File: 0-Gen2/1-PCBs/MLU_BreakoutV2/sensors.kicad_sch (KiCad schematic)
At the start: 6 parts, among them U2 MCP9808_MSOP, U3 MCP9808_MSOP, U4 BME280

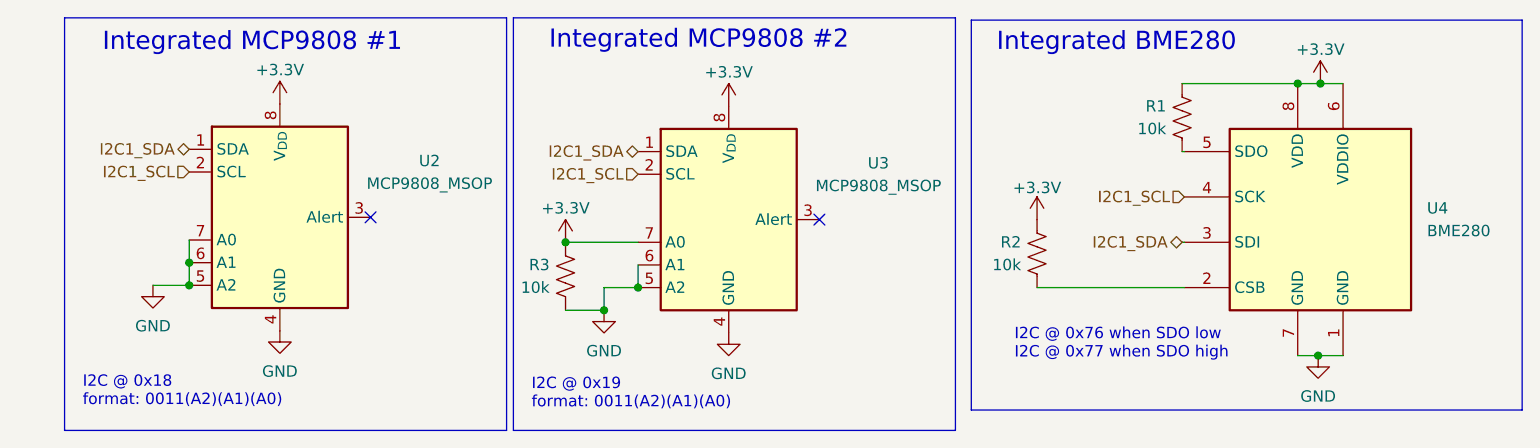
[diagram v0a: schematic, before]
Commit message: before restructure
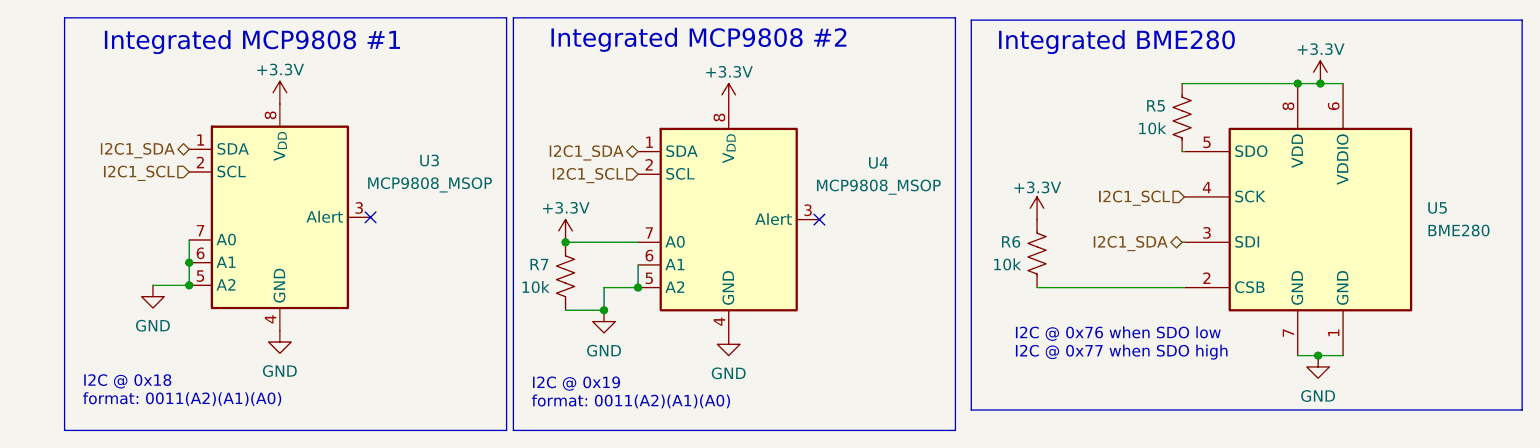
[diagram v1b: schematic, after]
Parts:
- renumbered R1 to R5, R2 to R6, R3 to R7, U2 to U3, U3 to U4, U4 to U5
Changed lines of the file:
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@@
 		(dnp no)
 		(fields_autoplaced yes)
-		(property "Reference" "#PWR021"
+		(property "Reference" "#PWR0145"
 			(at 93.472 59.182 0)
 			(effects
@@
 			(project "MLU_BreakoutV2"
 				(path "/55121ba7-5d22-4fe3-93aa-7f76d75b410c/9dab6a9b-c343-4374-86a4-2dd37d3a47bf"
-					(reference "#PWR021")
+					(reference "#PWR0145")
 					(unit 1)
 				)
@@
 		(dnp no)
 		(fields_autoplaced yes)
-		(property "Reference" "#PWR019"
+		(property "Reference" "#PWR0143"
 			(at 79.502 56.642 0)
 			(effects
@@
 			(project "MLU_BreakoutV2"
 				(path "/55121ba7-5d22-4fe3-93aa-7f76d75b410c/9dab6a9b-c343-4374-86a4-2dd37d3a47bf"
-					(reference "#PWR019")
+					(reference "#PWR0143")
 					(unit 1)
 				)
@@
 		(on_board yes)
 		(dnp no)
-		(property "Reference" "R2"
+		(property "Reference" "R6"
 			(at 126.238 42.6719 0)
 			(effects
@@
 			(project "MLU_BreakoutV2"
 				(path "/55121ba7-5d22-4fe3-93aa-7f76d75b410c/9dab6a9b-c343-4374-86a4-2dd37d3a47bf"
-					(reference "R2")
+					(reference "R6")
 					(unit 1)
 				)
@@
 		(on_board yes)
 		(dnp no)
-		(property "Reference" "#PWR012"
+		(property "Reference" "#PWR0138"
 			(at 43.18 30.988 0)
 			(effects
@@
 			(project "MLU_BreakoutV2"
 				(path "/55121ba7-5d22-4fe3-93aa-7f76d75b410c/9dab6a9b-c343-4374-86a4-2dd37d3a47bf"
-					(reference "#PWR012")
+					(reference "#PWR0138")
 					(unit 1)
 				)
@@
 		(dnp no)
 		(fields_autoplaced yes)
-		(property "Reference" "#PWR018"
+		(property "Reference" "#PWR0142"
 			(at 28.956 53.848 0)
 			(effects
@@
 			(project "MLU_BreakoutV2"
 				(path "/55121ba7-5d22-4fe3-93aa-7f76d75b410c/9dab6a9b-c343-4374-86a4-2dd37d3a47bf"
-					(reference "#PWR018")
+					(reference "#PWR0142")
 					(unit 1)
 				)
@@
 		(on_board yes)
 		(dnp no)
-		(property "Reference" "R3"
+		(property "Reference" "R7"
 			(at 73.406 45.2119 0)
 			(effects
@@
 			(project "MLU_BreakoutV2"
 				(path "/55121ba7-5d22-4fe3-93aa-7f76d75b410c/9dab6a9b-c343-4374-86a4-2dd37d3a47bf"
-					(reference "R3")
+					(reference "R7")
 					(unit 1)
 				)
@@
 		(dnp no)
 		(fields_autoplaced yes)
-		(property "Reference" "U2"
+		(property "Reference" "U3"
 			(at 59.944 33.5594 0)
 			(effects
@@
 			(project "MLU_BreakoutV2"
 				(path "/55121ba7-5d22-4fe3-93aa-7f76d75b410c/9dab6a9b-c343-4374-86a4-2dd37d3a47bf"
-					(reference "U2")
+					(reference "U3")
 					(unit 1)
 				)
@@
 		(on_board yes)
 		(dnp no)
-		(property "Reference" "U4"
+		(property "Reference" "U5"
 			(at 171.704 38.8619 0)
 			(effects
@@
 			(project "MLU_BreakoutV2"
 				(path "/55121ba7-5d22-4fe3-93aa-7f76d75b410c/9dab6a9b-c343-4374-86a4-2dd37d3a47bf"
-					(reference "U4")
+					(reference "U5")
 					(unit 1)
 				)
@@
 		(on_board yes)
 		(dnp no)
-		(property "Reference" "#PWR017"
+		(property "Reference" "#PWR0141"
 			(at 75.184 46.482 0)
 			(effects
@@
 			(project "MLU_BreakoutV2"
 				(path "/55121ba7-5d22-4fe3-93aa-7f76d75b410c/9dab6a9b-c343-4374-86a4-2dd37d3a47bf"
-					(reference "#PWR017")
+					(reference "#PWR0141")
 					(unit 1)
 				)
@@
 		(dnp no)
 		(fields_autoplaced yes)
-		(property "Reference" "#PWR022"
+		(property "Reference" "#PWR0146"
 			(at 159.512 61.722 0)
 			(effects
@@
 			(project "MLU_BreakoutV2"
 				(path "/55121ba7-5d22-4fe3-93aa-7f76d75b410c/9dab6a9b-c343-4374-86a4-2dd37d3a47bf"
-					(reference "#PWR022")
+					(reference "#PWR0146")
 					(unit 1)
 				)
@@
 		(dnp no)
 		(fields_autoplaced yes)
-		(property "Reference" "U3"
+		(property "Reference" "U4"
 			(at 110.236 33.8134 0)
 			(effects
@@
 			(project "MLU_BreakoutV2"
 				(path "/55121ba7-5d22-4fe3-93aa-7f76d75b410c/9dab6a9b-c343-4374-86a4-2dd37d3a47bf"
-					(reference "U3")
+					(reference "U4")
 					(unit 1)
 				)
@@
 		(on_board yes)
 		(dnp no)
-		(property "Reference" "#PWR09"
+		(property "Reference" "#PWR0137"
 			(at 159.766 28.702 0)
 			(effects
@@
 			(project "MLU_BreakoutV2"
 				(path "/55121ba7-5d22-4fe3-93aa-7f76d75b410c/9dab6a9b-c343-4374-86a4-2dd37d3a47bf"
-					(reference "#PWR09")
+					(reference "#PWR0137")
 					(unit 1)
 				)
@@
 		(on_board yes)
 		(dnp no)
-		(property "Reference" "#PWR014"
+		(property "Reference" "#PWR0140"
 			(at 128.016 43.942 0)
 			(effects
@@
 			(project "MLU_BreakoutV2"
 				(path "/55121ba7-5d22-4fe3-93aa-7f76d75b410c/9dab6a9b-c343-4374-86a4-2dd37d3a47bf"
-					(reference "#PWR014")
+					(reference "#PWR0140")
 					(unit 1)
 				)
@@
 		(on_board yes)
 		(dnp no)
-		(property "Reference" "R1"
+		(property "Reference" "R5"
 			(at 142.494 27.4319 0)
 			(effects
@@
 			(project "MLU_BreakoutV2"
 				(path "/55121ba7-5d22-4fe3-93aa-7f76d75b410c/9dab6a9b-c343-4374-86a4-2dd37d3a47bf"
-					(reference "R1")
+					(reference "R5")
 					(unit 1)
 				)
@@
 		(on_board yes)
 		(dnp no)
-		(property "Reference" "#PWR013"
+		(property "Reference" "#PWR0139"
 			(at 93.472 31.242 0)
 			(effects
@@
 			(project "MLU_BreakoutV2"
 				(path "/55121ba7-5d22-4fe3-93aa-7f76d75b410c/9dab6a9b-c343-4374-86a4-2dd37d3a47bf"
-					(reference "#PWR013")
+					(reference "#PWR0139")
 					(unit 1)
 				)
@@
 		(dnp no)
 		(fields_autoplaced yes)
-		(property "Reference" "#PWR020"
+		(property "Reference" "#PWR0144"
 			(at 43.18 58.928 0)
 			(effects
@@
 			(project "MLU_BreakoutV2"
 				(path "/55121ba7-5d22-4fe3-93aa-7f76d75b410c/9dab6a9b-c343-4374-86a4-2dd37d3a47bf"
-					(reference "#PWR020")
-					(unit 1)
-				)
+					(reference "#PWR0144")
+					(unit 1)
+				)
